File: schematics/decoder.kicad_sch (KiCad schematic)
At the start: 4 parts, among them U10 ATF22V10C-7, U11 74HC373, U29 74HC245, U9 ATF22V10C-7

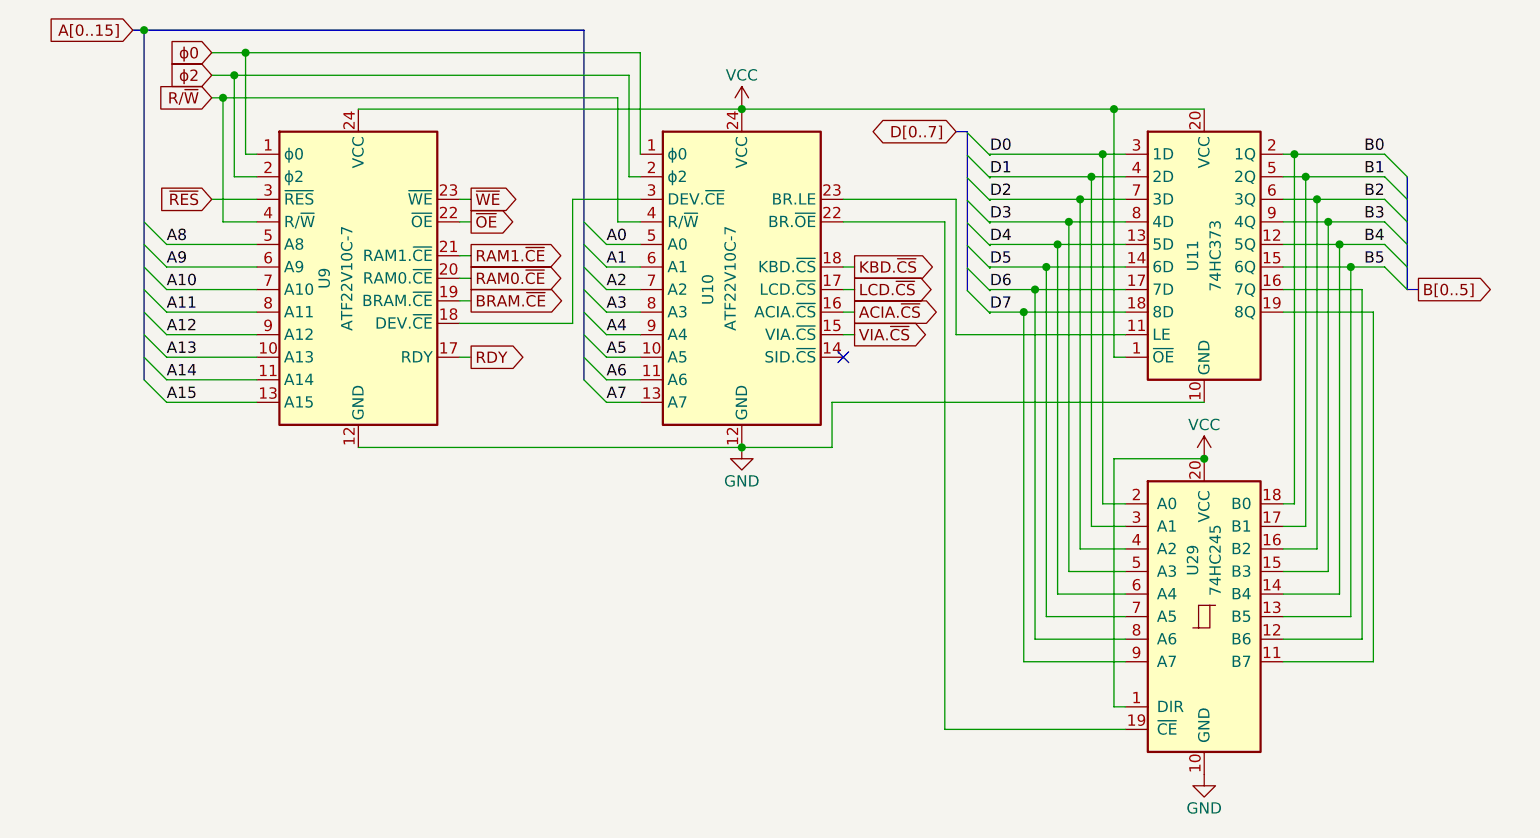
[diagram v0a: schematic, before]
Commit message: fixing wiring
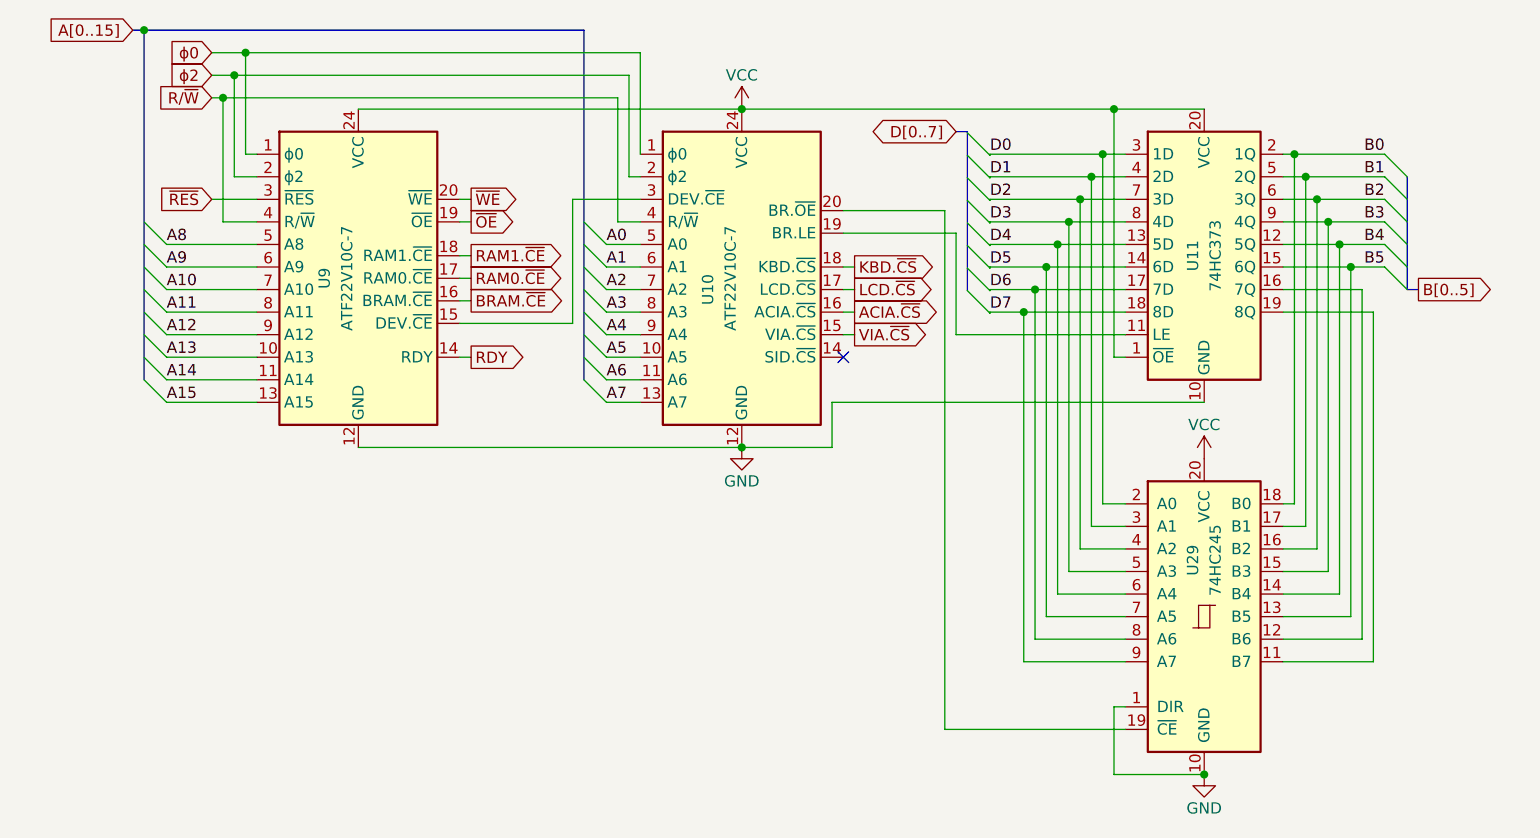
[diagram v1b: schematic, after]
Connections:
- net BRAM.~{CE}: now also U9.16 (BRAM.~{CE}); no longer U9.19 (BRAM.~{CE})
- net GND: now also U29.1 (DIR)
- net RAM0.~{CE}: now also U9.17 (RAM0.~{CE}); no longer U9.20 (RAM0.~{CE})
- net RAM1.~{CE}: now also U9.18 (RAM1.~{CE}); no longer U9.21 (RAM1.~{CE})
- net RDY: now also U9.14 (RDY); no longer U9.17 (RDY)
- net VCC: no longer U29.1 (DIR)
- net ~{OE}: now also U9.19 (~{OE}); no longer U9.22 (~{OE})
- net ~{WE}: now also U9.20 (~{WE}); no longer U9.23 (~{WE})
- net at U11.11 (LE): now also U10.19 (BR.LE); no longer U10.23 (BR.LE)
- net at U10.20 (BR.~{OE}): now also U29.19 (~{CE})
- net at U10.22: no longer U29.19 (~{CE})
- net at U10.3 (DEV.~{CE}): now also U9.15 (DEV.~{CE}); no longer U9.18 (DEV.~{CE})
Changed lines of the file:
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@@
+	)
+	(junction
+		(at 186.69 143.51)
+		(diameter 0)
+		(color 0 0 0 0)
 	)
 	(junction
@@
 	(junction
 		(at 201.93 83.82)
-		(diameter 0)
-		(color 0 0 0 0)
-	)
-	(junction
-		(at 186.69 107.95)
 		(diameter 0)
 		(color 0 0 0 0)
@@
 	(wire
 		(pts
+			(xy 176.53 143.51) (xy 186.69 143.51)
+		)
+		(stroke
+			(width 0)
+			(type default)
+		)
+	)
+	(wire
+		(pts
 			(xy 162.56 76.2) (xy 173.99 76.2)
 		)
@@
 	(wire
 		(pts
-			(xy 176.53 107.95) (xy 186.69 107.95)
-		)
-		(stroke
-			(width 0)
-			(type default)
-		)
-	)
-	(wire
-		(pts
 			(xy 171.45 81.28) (xy 177.8 81.28)
 		)
@@
 	(wire
 		(pts
-			(xy 176.53 135.89) (xy 176.53 107.95)
-		)
-		(stroke
-			(width 0)
-			(type default)
-		)
-	)
-	(wire
-		(pts
 			(xy 177.8 130.81) (xy 166.37 130.81)
 		)
@@
 	(wire
 		(pts
-			(xy 158.75 78.74) (xy 146.05 78.74)
-		)
-		(stroke
-			(width 0)
-			(type default)
-		)
-	)
-	(wire
-		(pts
-			(xy 146.05 81.28) (xy 157.48 81.28)
+			(xy 158.75 82.55) (xy 146.05 82.55)
+		)
+		(stroke
+			(width 0)
+			(type default)
+		)
+	)
+	(wire
+		(pts
+			(xy 146.05 80.01) (xy 157.48 80.01)
 		)
 		(stroke
@@
 	(wire
 		(pts
-			(xy 157.48 81.28) (xy 157.48 138.43)
+			(xy 157.48 80.01) (xy 157.48 138.43)
 		)
 		(stroke
@@
 	(wire
 		(pts
-			(xy 158.75 93.98) (xy 158.75 78.74)
+			(xy 158.75 93.98) (xy 158.75 82.55)
 		)
 		(stroke
@@
 		)
 		(stroke
+			(width 0)
+			(type default)
+		)
+	)
+	(wire
+		(pts
+			(xy 176.53 135.89) (xy 176.53 143.51)
+		)
+		(stroke
